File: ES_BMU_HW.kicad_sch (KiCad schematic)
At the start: 22 parts, among them J1 Conn_02x02_Top_Bottom, J2 Conn_02x02_Top_Bottom, J3 Conn_02x03_Top_Bottom, J4 Conn_02x06_Top_Bottom, J6 Conn_02x04_Top_Bottom, U1 TPS542025, U7 TLV777

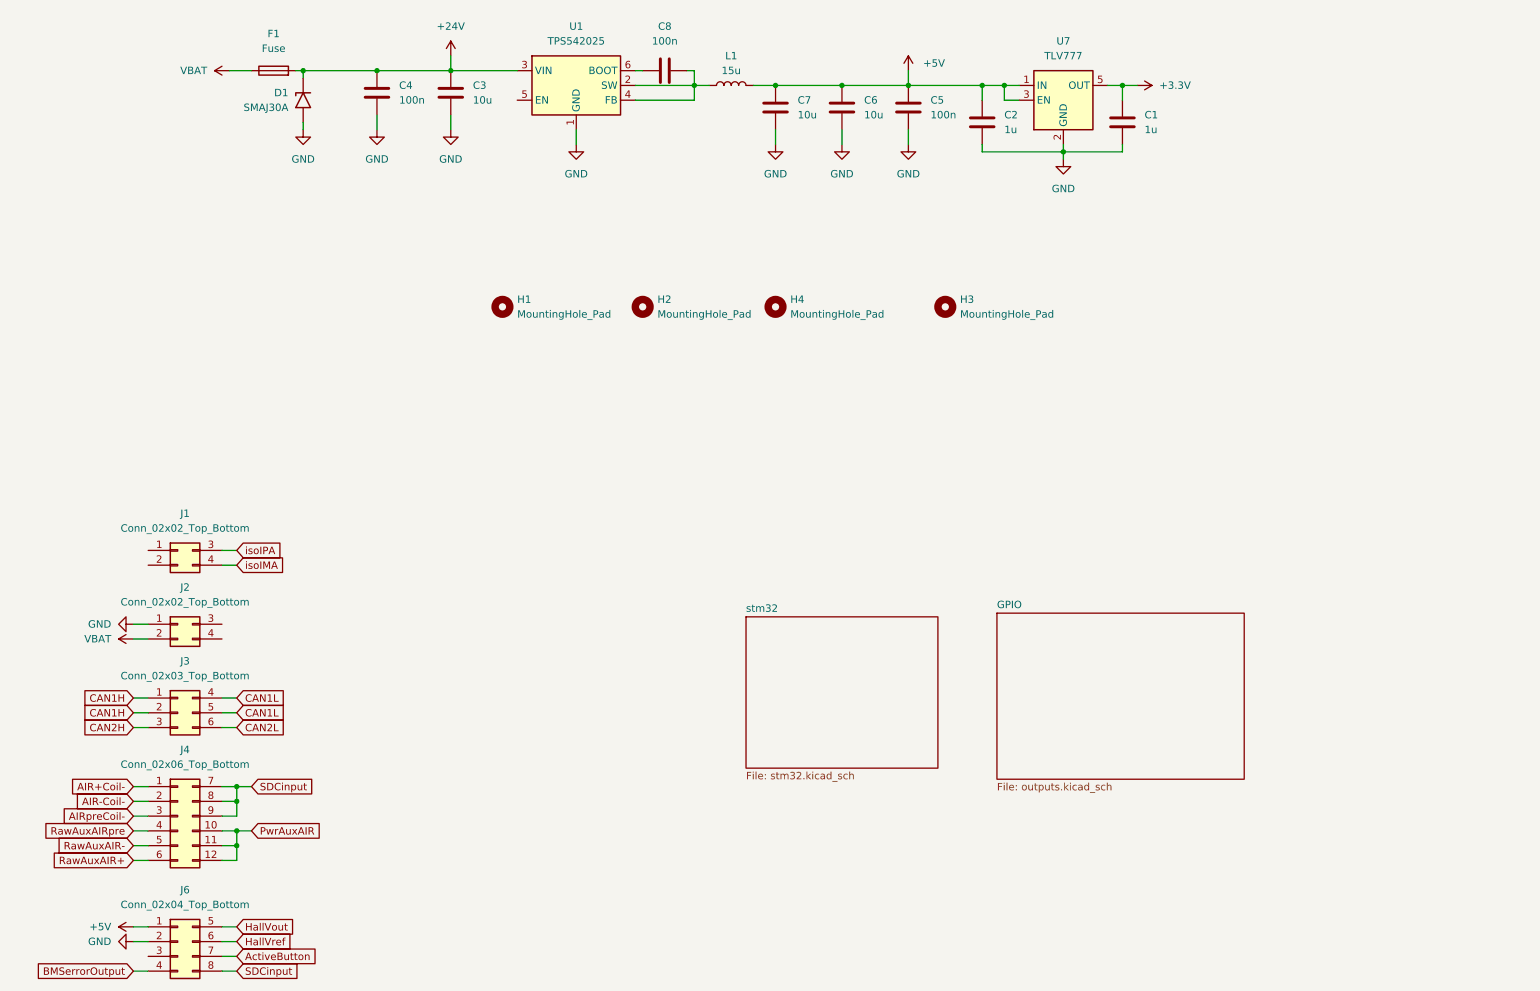
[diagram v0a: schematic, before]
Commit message: updated schematics template
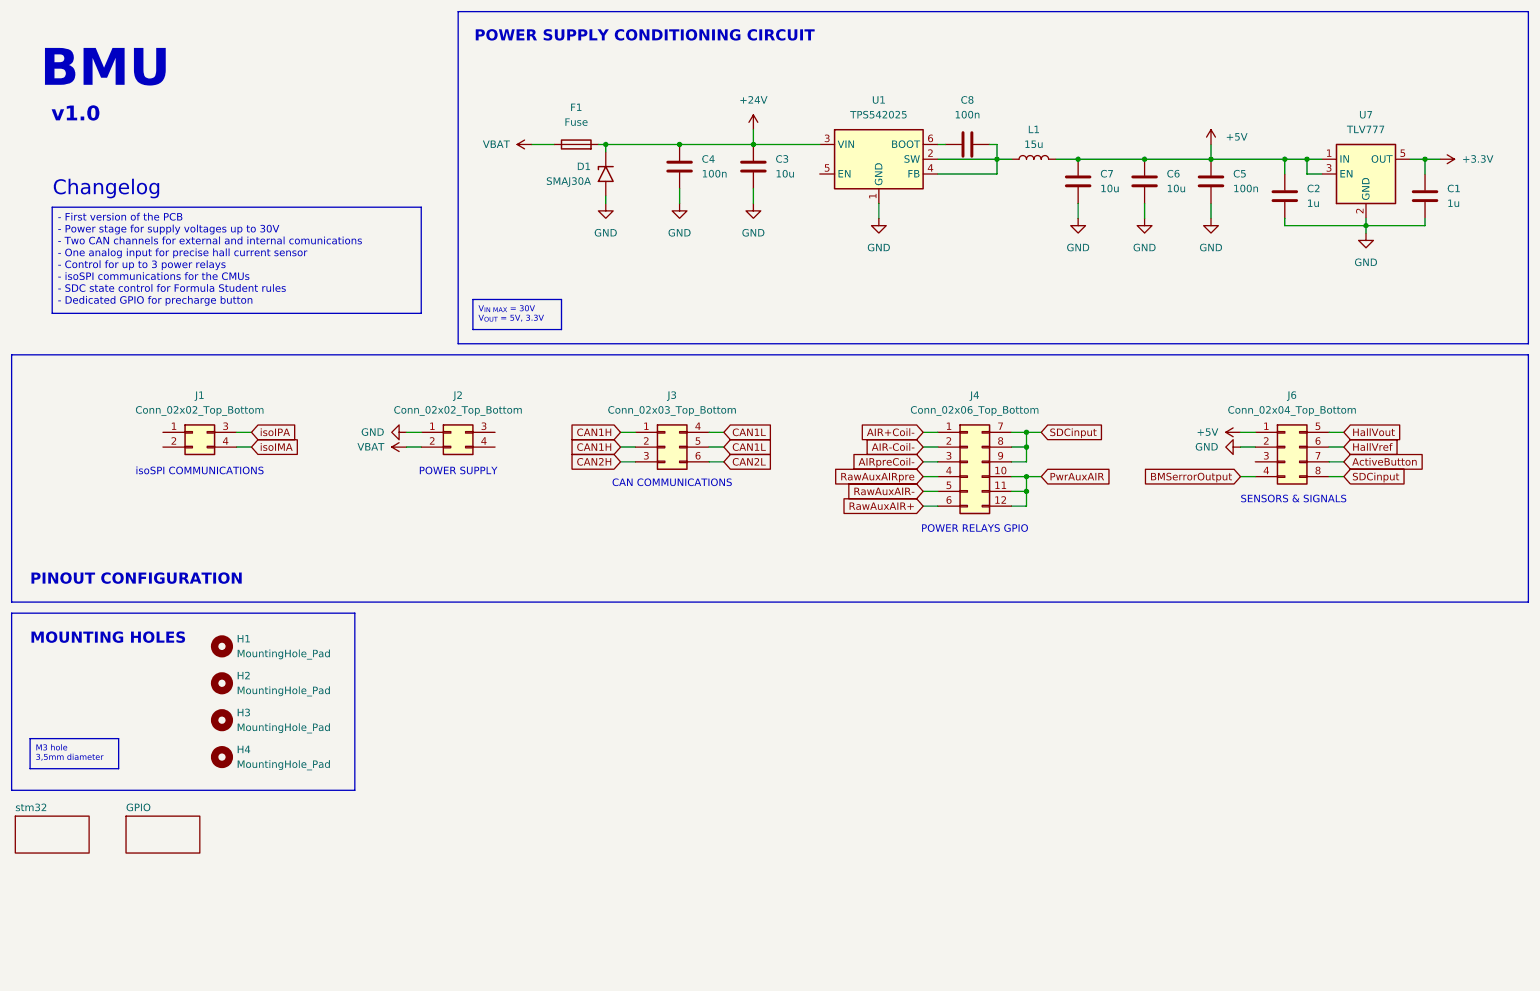
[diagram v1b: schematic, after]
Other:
- note added: "BMU"
- note added: "CAN COMMUNICATIONS"
- note added: "Changelog"
- note added: "MOUNTING HOLES"
- note added: "PINOUT CONFIGURATION"
- note added: "POWER RELAYS GPIO"
- note added: "POWER SUPPLY"
- note added: "POWER SUPPLY CONDITIONING CIRCUIT"
- note added: "SENSORS & SIGNALS"
- note added: "isoSPI COMMUNICATIONS"
- note added: "v1.0"
- company: (none) -> EUSS Motorsport
- title: (none) -> BMU
- moved on the sheet: C1, C2, C3, C4, C5, C6, C7, C8, D1, F1, H1, H2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
